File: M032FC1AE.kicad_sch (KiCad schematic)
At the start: 21 parts, among them IC1 M032FC1AE, J1 Conn_01x10, J2 Conn_01x03, J3 Conn_01x04, Q1 S8050, SW1 SW_Push, SW2 SW_Slide_DPDT, U1 AMS1117-1.8, U2 AMS1117-3.3

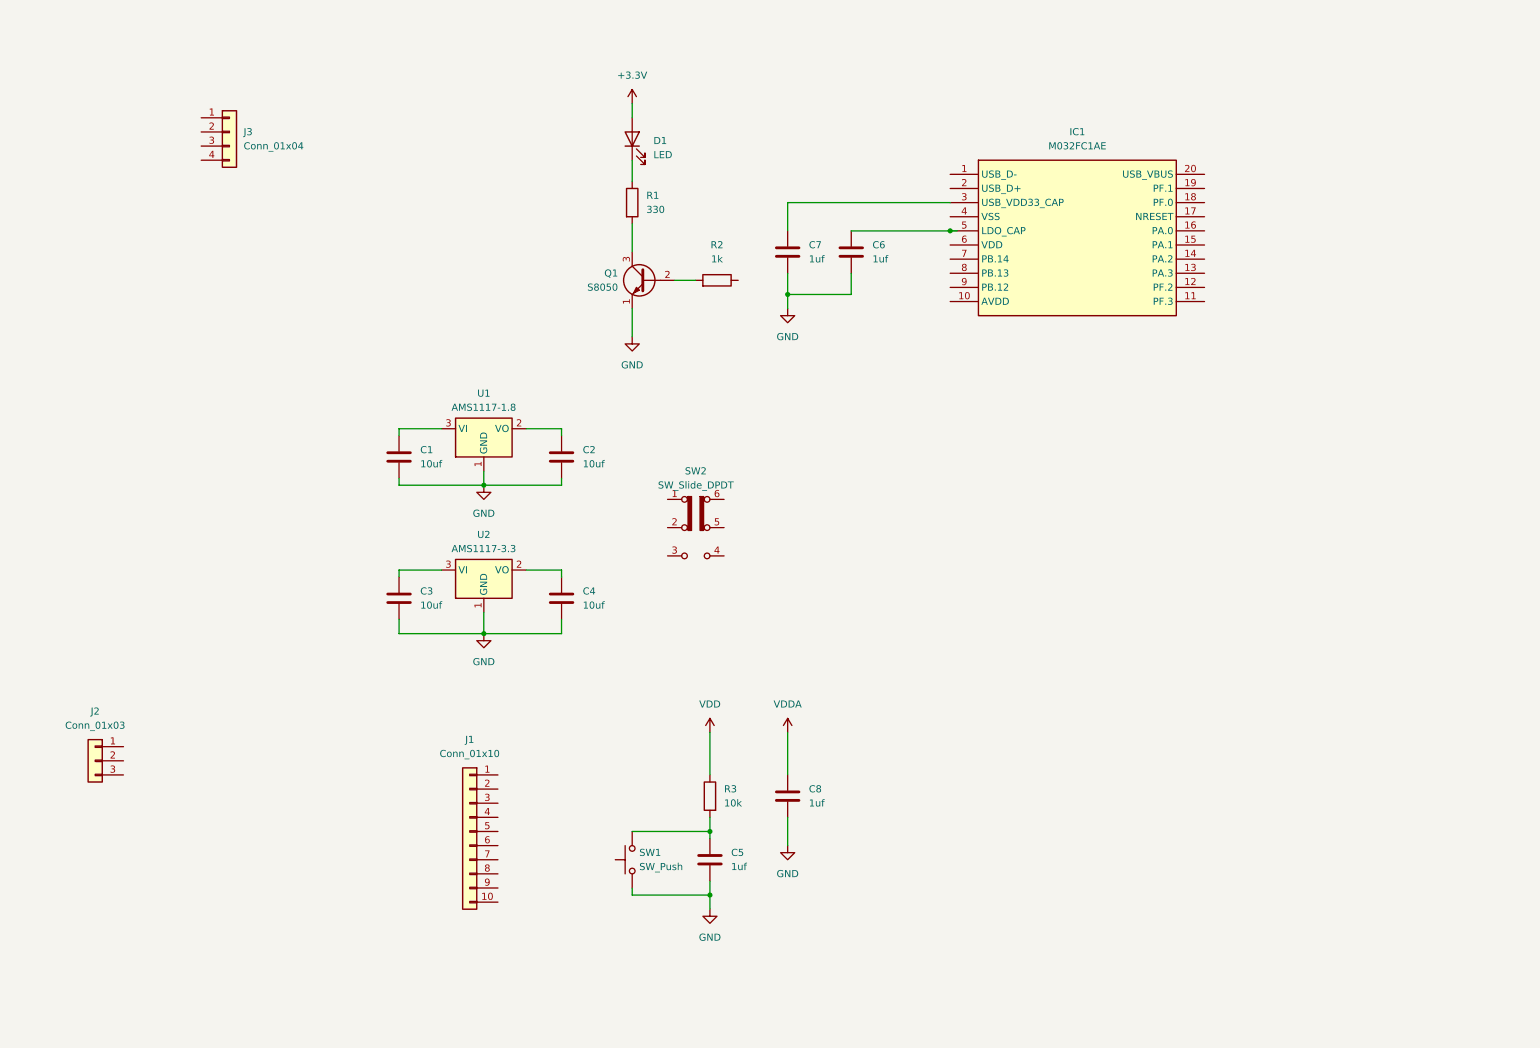
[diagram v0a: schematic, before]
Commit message: Update Modify
Change-Id: I51f3ca84c8081b6ca1092425d51957d997ef9c07
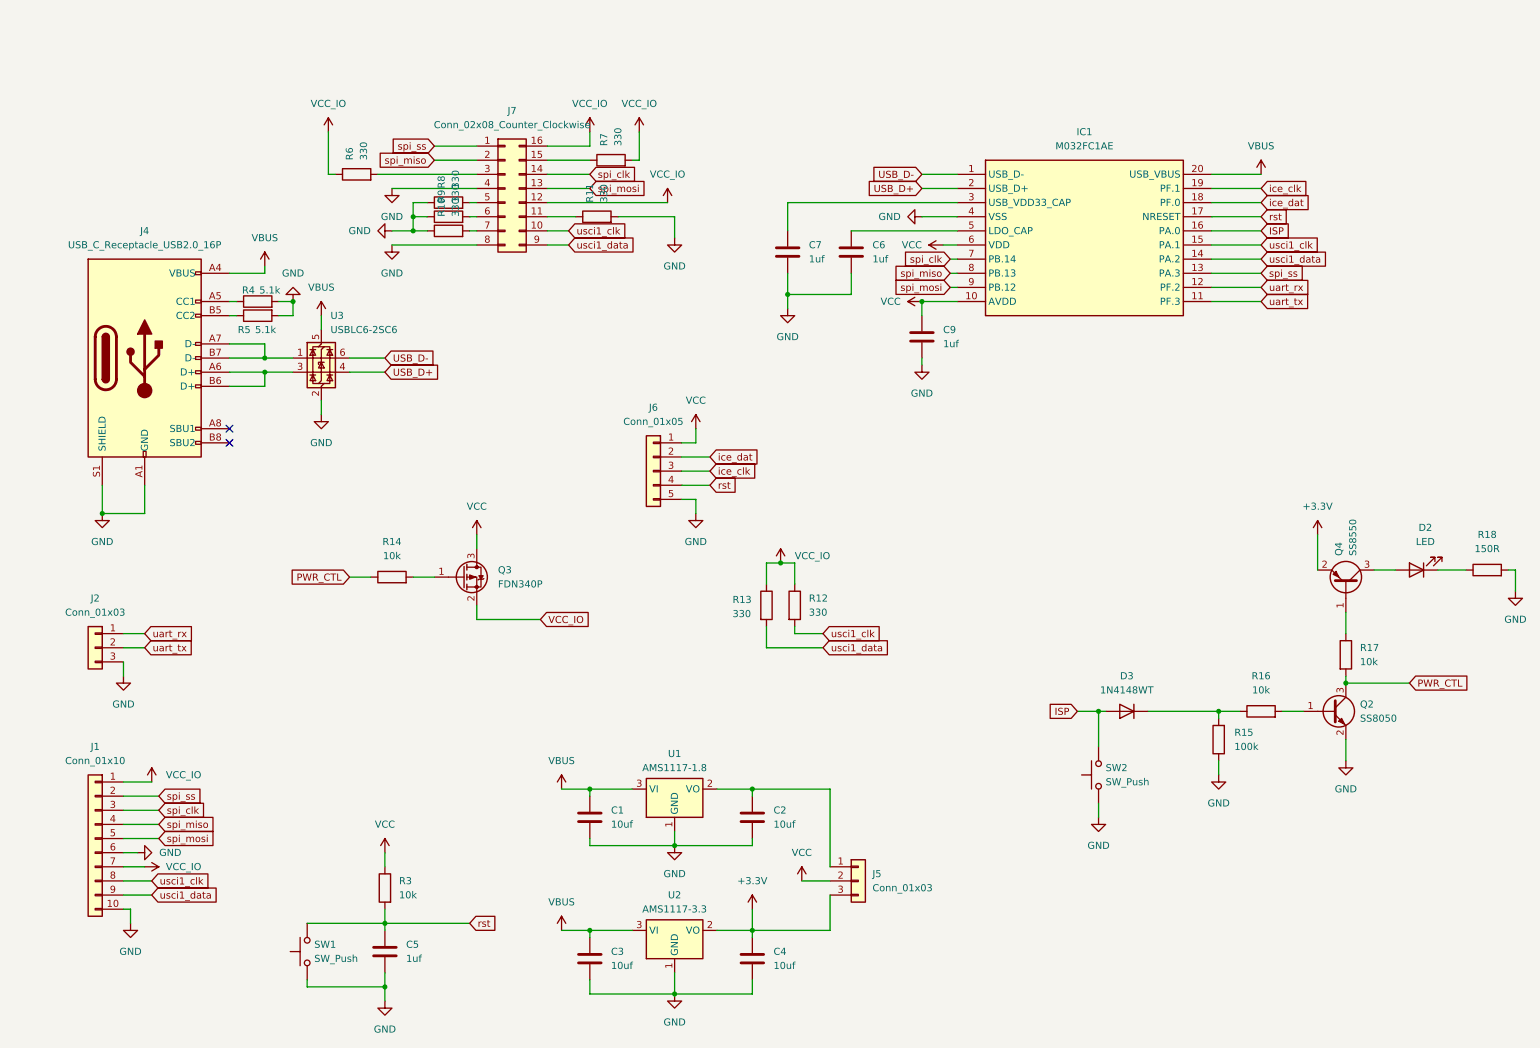
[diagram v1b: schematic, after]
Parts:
- removed C8: 1uf, Capacitor_SMD:C_0603_1608Metric_Pad1.08x0.95mm_HandSolder, symbol Device:C
- removed D1: LED, LED_THT:LED_D3.0mm, symbol Device:LED
- removed J3: Conn_01x04, Connector_PinHeader_2.54mm:PinHeader_1x04_P2.54mm_Horizontal, symbol Connector_Generic:Conn_01x04
- removed Q1: S8050, Package_TO_SOT_THT:TO-92_Inline, symbol Transistor_BJT:S8050
- removed R1: 330, Resistor_SMD:R_0603_1608Metric_Pad0.98x0.95mm_HandSolder, symbol Device:R
- removed R2: 1k, Resistor_SMD:R_0603_1608Metric_Pad0.98x0.95mm_HandSolder, symbol Device:R
- removed SW2: SW_Slide_DPDT, Button_Switch_THT:SW_E-Switch_EG2219_DPDT_Angled, symbol Switch:SW_Slide_DPDT
- added C9: 1uf, Capacitor_SMD:C_0603_1608Metric_Pad1.08x0.95mm_HandSolder, symbol Device:C
- added D2: LED, LED_THT:LED_D3.0mm, symbol Device:LED
- added D3: 1N4148WT, Diode_SMD:D_SOD-523, symbol Diode:1N4148WT
- added J4: USB_C_Receptacle_USB2.0_16P, Connector_USB:USB_C_Receptacle_GCT_USB4105-xx-A_16P_TopMnt_Horizontal, symbol Connector:USB_C_Receptacle_USB2.0_16P
- added J5: Conn_01x03, Connector_PinHeader_2.54mm:PinHeader_1x03_P2.54mm_Vertical, symbol Connector_Generic:Conn_01x03
- added J6: Conn_01x05, Connector_PinSocket_2.54mm:PinSocket_1x05_P2.54mm_Horizontal, symbol Connector_Generic:Conn_01x05
- added J7: Conn_02x08_Counter_Clockwise, Socket:DIP_Socket-16_W4.3_W5.08_W7.62_W10.16_W10.9_3M_216-3340-00-0602J, symbol Connector_Generic:Conn_02x08_Counter_Clockwise
- added Q2: SS8050, Package_TO_SOT_SMD:SOT-23, symbol Transistor_BJT:SS8050
- added Q3: FDN340P, Package_TO_SOT_SMD:SOT-23, symbol Transistor_FET:FDN340P
- added Q4: SS8550, Package_TO_SOT_SMD:SOT-23, symbol Transistor_BJT:SS8550
- added R10, R11, R12, R13, R6, R7, R8, R9: 330, Resistor_SMD:R_0603_1608Metric_Pad0.98x0.95mm_HandSolder, symbol Device:R
- added R14, R16, R17: 10k, Resistor_SMD:R_0603_1608Metric_Pad0.98x0.95mm_HandSolder, symbol Device:R
- added R15: 100k, Resistor_SMD:R_0603_1608Metric_Pad0.98x0.95mm_HandSolder, symbol Device:R
- added R18: 150R, Resistor_SMD:R_0603_1608Metric_Pad0.98x0.95mm_HandSolder, symbol Device:R
- added R4, R5: 5.1k, Resistor_SMD:R_0603_1608Metric_Pad0.98x0.95mm_HandSolder, symbol Device:R
- added SW2: SW_Push, Button_Switch_THT:SW_PUSH_6mm, symbol Switch:SW_Push
- added U3: USBLC6-2SC6, Package_TO_SOT_SMD:SOT-23-6, symbol Power_Protection:USBLC6-2SC6
- IC1: footprint SOP65P640X120-20N -> M032FC1AE:M032FC1AE
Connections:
- net VDD is gone; now on net VCC: R3.1
- net +3.3V: now also C4.1, U2.2 (VO), J5.3 (Pin_3), Q4.2 (E)
- net GND: now also IC1.4 (VSS), J1.10 (Pin_10), J1.6 (Pin_6), J2.3 (Pin_3), C9.2, J4.A1 (GND), J4.A12 (GND), J4.B1 (GND), J4.B12 (GND), J4.S1 (SHIELD), J6.5 (Pin_5), J7.4 (Pin_4), J7.8 (Pin_8), Q2.2 (E), R10.1, R11.2, R15.1, R18.2, R4.2, R5.2, R8.1, R9.1, SW2.1, U3.2 (GND)
- net rst: now reaches C5.1, R3.2, SW1.2
- net rst: now also IC1.17 (NRESET), J6.4 (Pin_4)
- net VBUS: now reaches C3.1, U2.3 (VI)
- net VBUS: now also C1.1, IC1.20 (USB_VBUS), U1.3 (VI), J4.A4 (VBUS), J4.A9 (VBUS), J4.B4 (VBUS), J4.B9 (VBUS), U3.5 (VBUS)
- net uart_rx: now reaches J2.1 (Pin_1)
- net uart_rx: now also IC1.12 (PF.2)
- net uart_tx: now reaches J2.2 (Pin_2)
- net uart_tx: now also IC1.11 (PF.3)
- net USB_D-: now reaches IC1.1 (USB_D-)
- net USB_D-: now also U3.6 (I/O1)
- net VCC: now reaches IC1.10 (AVDD)
- net VCC: now also IC1.6 (VDD), C9.1, J5.2 (Pin_2), J6.1 (Pin_1), Q3.3 (D)
- net spi_ss: now reaches IC1.13 (PA.3)
- net spi_ss: now also J1.2 (Pin_2), J7.1 (Pin_1)
- net usci1_data: now reaches IC1.14 (PA.2)
- net usci1_data: now also J1.9 (Pin_9), J7.9 (Pin_9), R13.2
- net usci1_clk: now reaches IC1.15 (PA.1)
- net usci1_clk: now also J1.8 (Pin_8), J7.10 (Pin_10), R12.2
- net ISP: now reaches IC1.16 (PA.0)
- net ISP: now also D3.2 (A), SW2.2
- net ice_dat: now reaches IC1.18 (PF.0)
- net ice_dat: now also J6.2 (Pin_2)
- net ice_clk: now reaches IC1.19 (PF.1)
- net ice_clk: now also J6.3 (Pin_3)
- net USB_D+: now reaches IC1.2 (USB_D+)
- net USB_D+: now also U3.4 (I/O2)
- net spi_clk: now reaches IC1.7 (PB.14)
- net spi_clk: now also J1.3 (Pin_3), J7.14 (Pin_14)
- net spi_miso: now reaches IC1.8 (PB.13)
- net spi_miso: now also J1.4 (Pin_4), J7.2 (Pin_2)
- net spi_mosi: now reaches IC1.9 (PB.12)
- net spi_mosi: now also J1.5 (Pin_5), J7.13 (Pin_13)
- net at C2.1, U1.2 (VO): now also J5.1 (Pin_1)
- net VCC_IO: now reaches J1.1 (Pin_1)
- net VCC_IO: now also J1.7 (Pin_7), J7.12 (Pin_12), J7.16 (Pin_16), Q3.2 (S), R12.1, R13.1, R6.1, R7.2
- new net: J7.11 (Pin_11), R11.1
- new net: J7.15 (Pin_15), R7.1
- new net: J7.3 (Pin_3), R6.2
- new net: J7.5 (Pin_5), R8.2
- new net: J7.6 (Pin_6), R9.2
- new net: J7.7 (Pin_7), R10.2
- new net: Q3.1 (G), R14.2
- new net: J4.A7 (D-), J4.B7 (D-), U3.1 (I/O1)
- new net: J4.A6 (D+), J4.B6 (D+), U3.3 (I/O2)
- new net: D2.1 (K), R18.1
- new net: D2.2 (A), Q4.3 (C)
- new net: Q2.1 (B), R16.2
- new net: D3.1 (K), R15.2, R16.1
- new net: J4.A5 (CC1), R4.1
- new net: Q4.1 (B), R17.1
- new net: J4.B5 (CC2), R5.1
- new net PWR_CTL: Q2.3 (C), R14.1, R17.2
- no-connect marks 0 -> 2
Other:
- moved on the sheet: C1, C2, C3, C4, C5, IC1, J1, J2, R3, SW1, U1, U2

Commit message: Release Gerver V0.1
Change-Id: If113fa1b5dadd0f7a6d01bb5205053d055243908
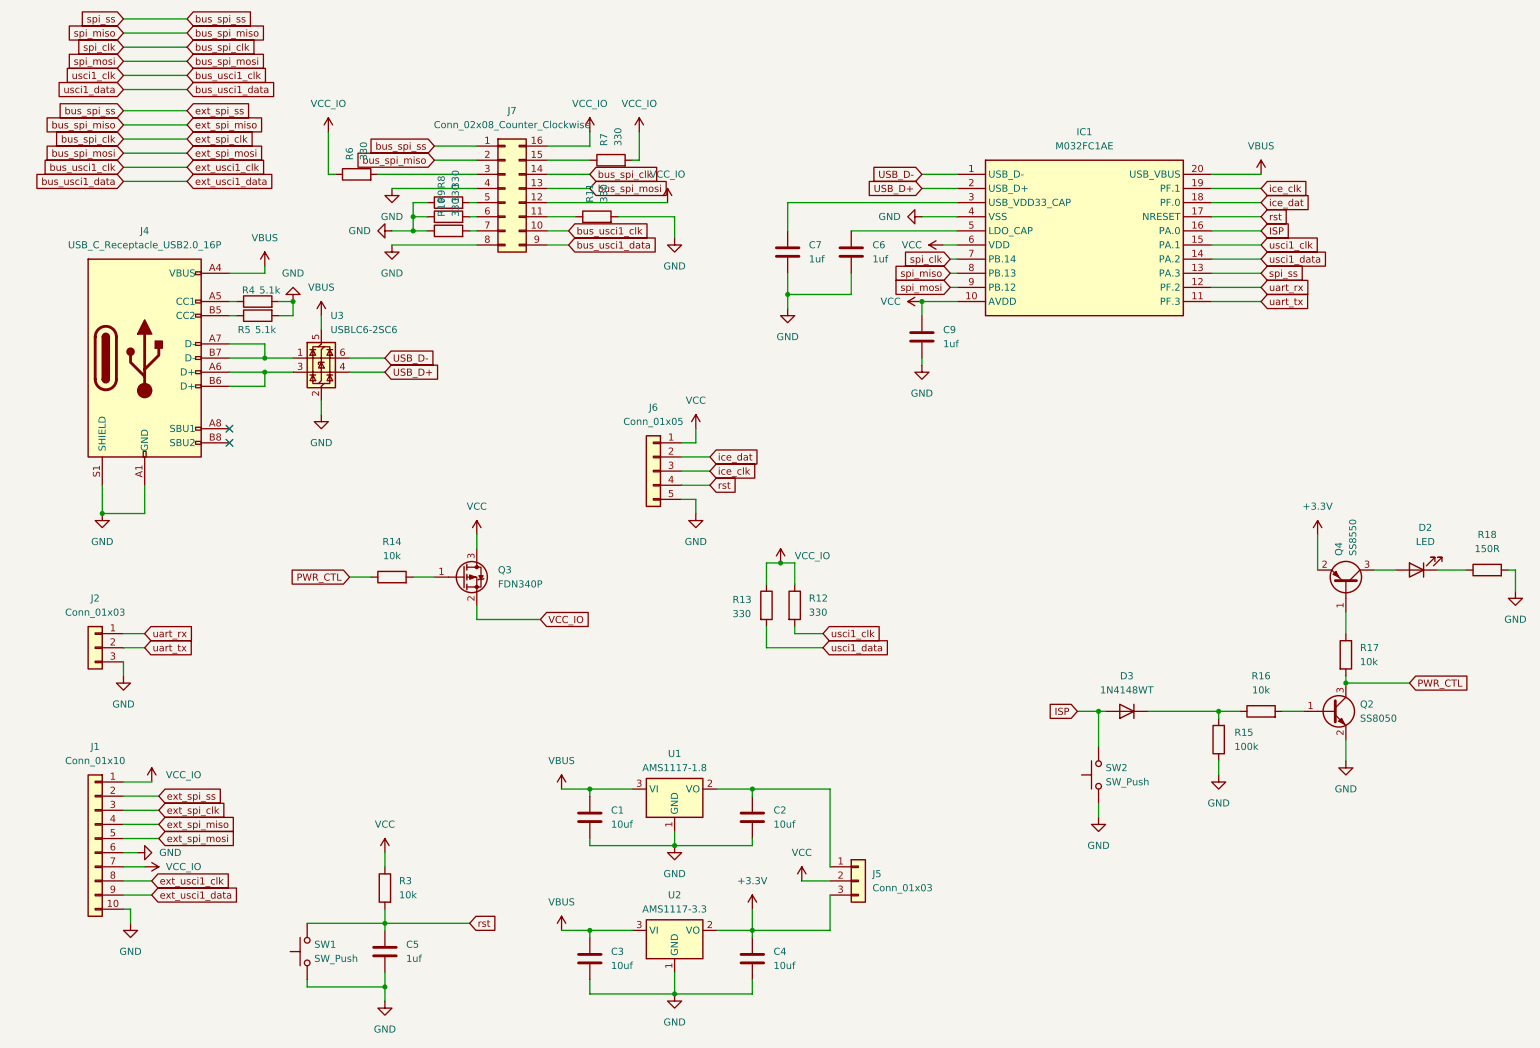
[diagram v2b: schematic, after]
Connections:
- net spi_clk renamed bus_spi_clk
- net spi_miso renamed bus_spi_miso
- net spi_mosi renamed bus_spi_mosi
- net spi_ss renamed bus_spi_ss
- net usci1_clk renamed bus_usci1_clk
- net usci1_data renamed bus_usci1_data
